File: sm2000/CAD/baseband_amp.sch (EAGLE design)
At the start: 20 parts, among them Q1 BC548, Q4 BC549

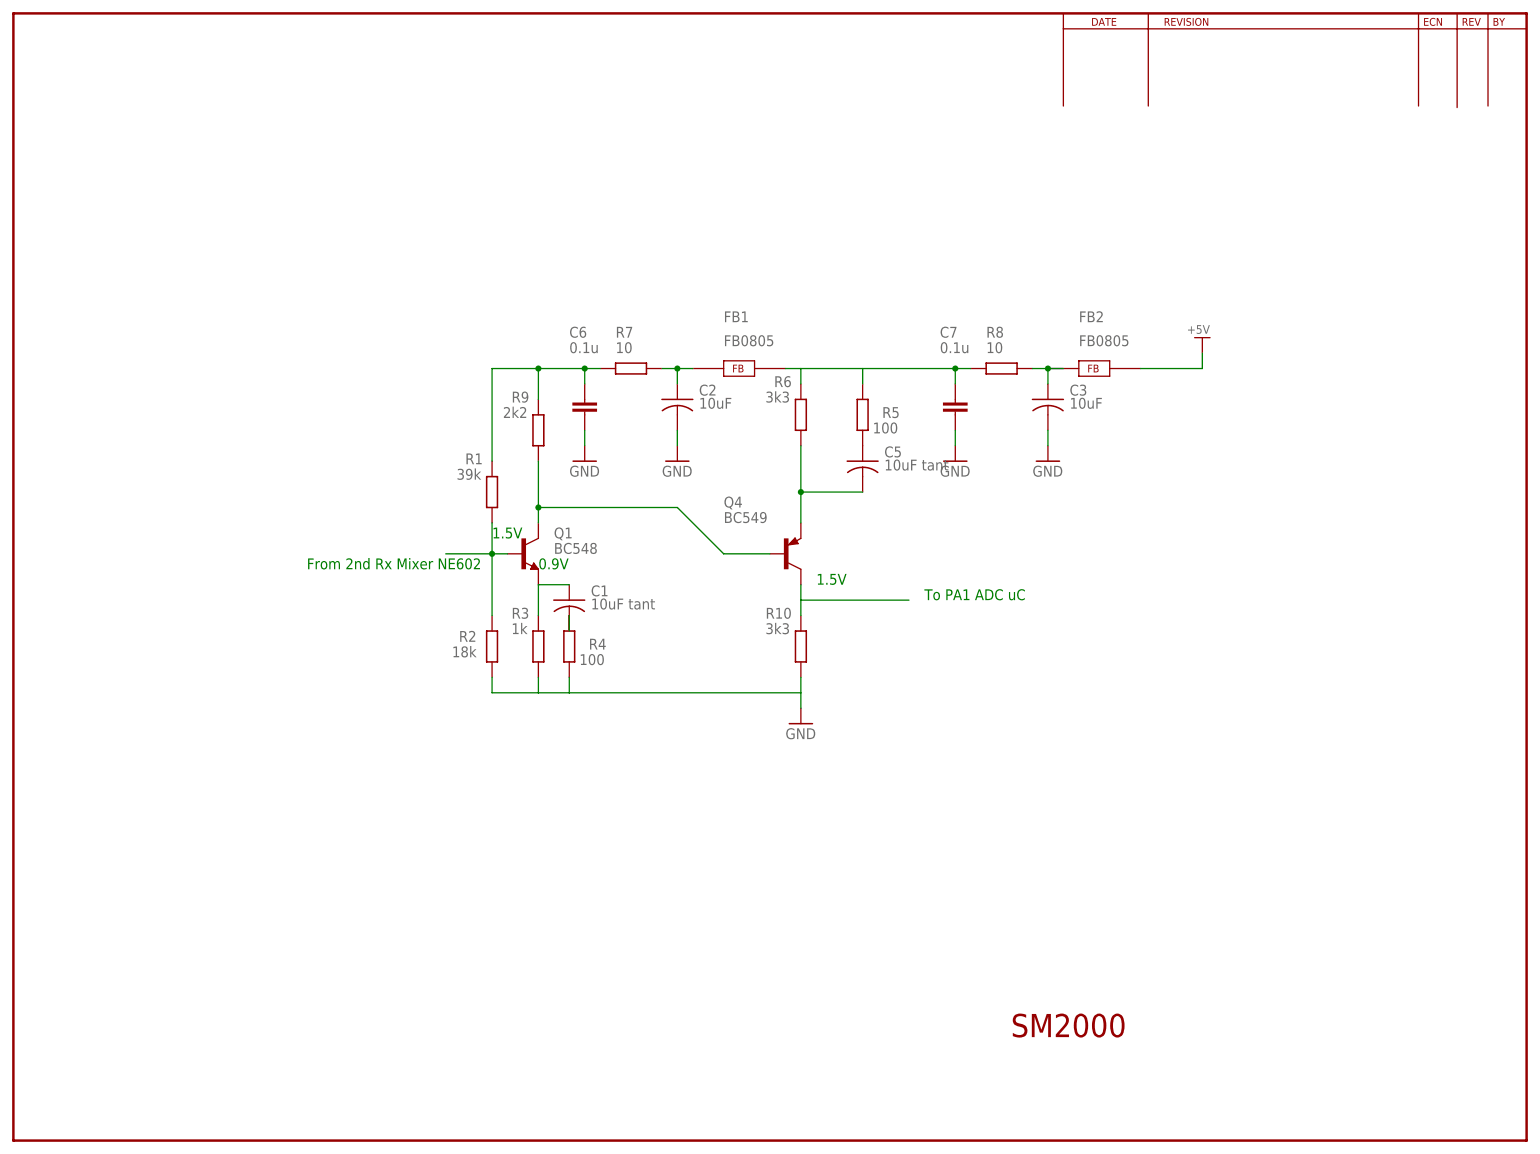
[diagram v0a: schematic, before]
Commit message: COMMIT SM2000 SCHEMATIC, PCB AND ADDED PART DOCS.  RGB
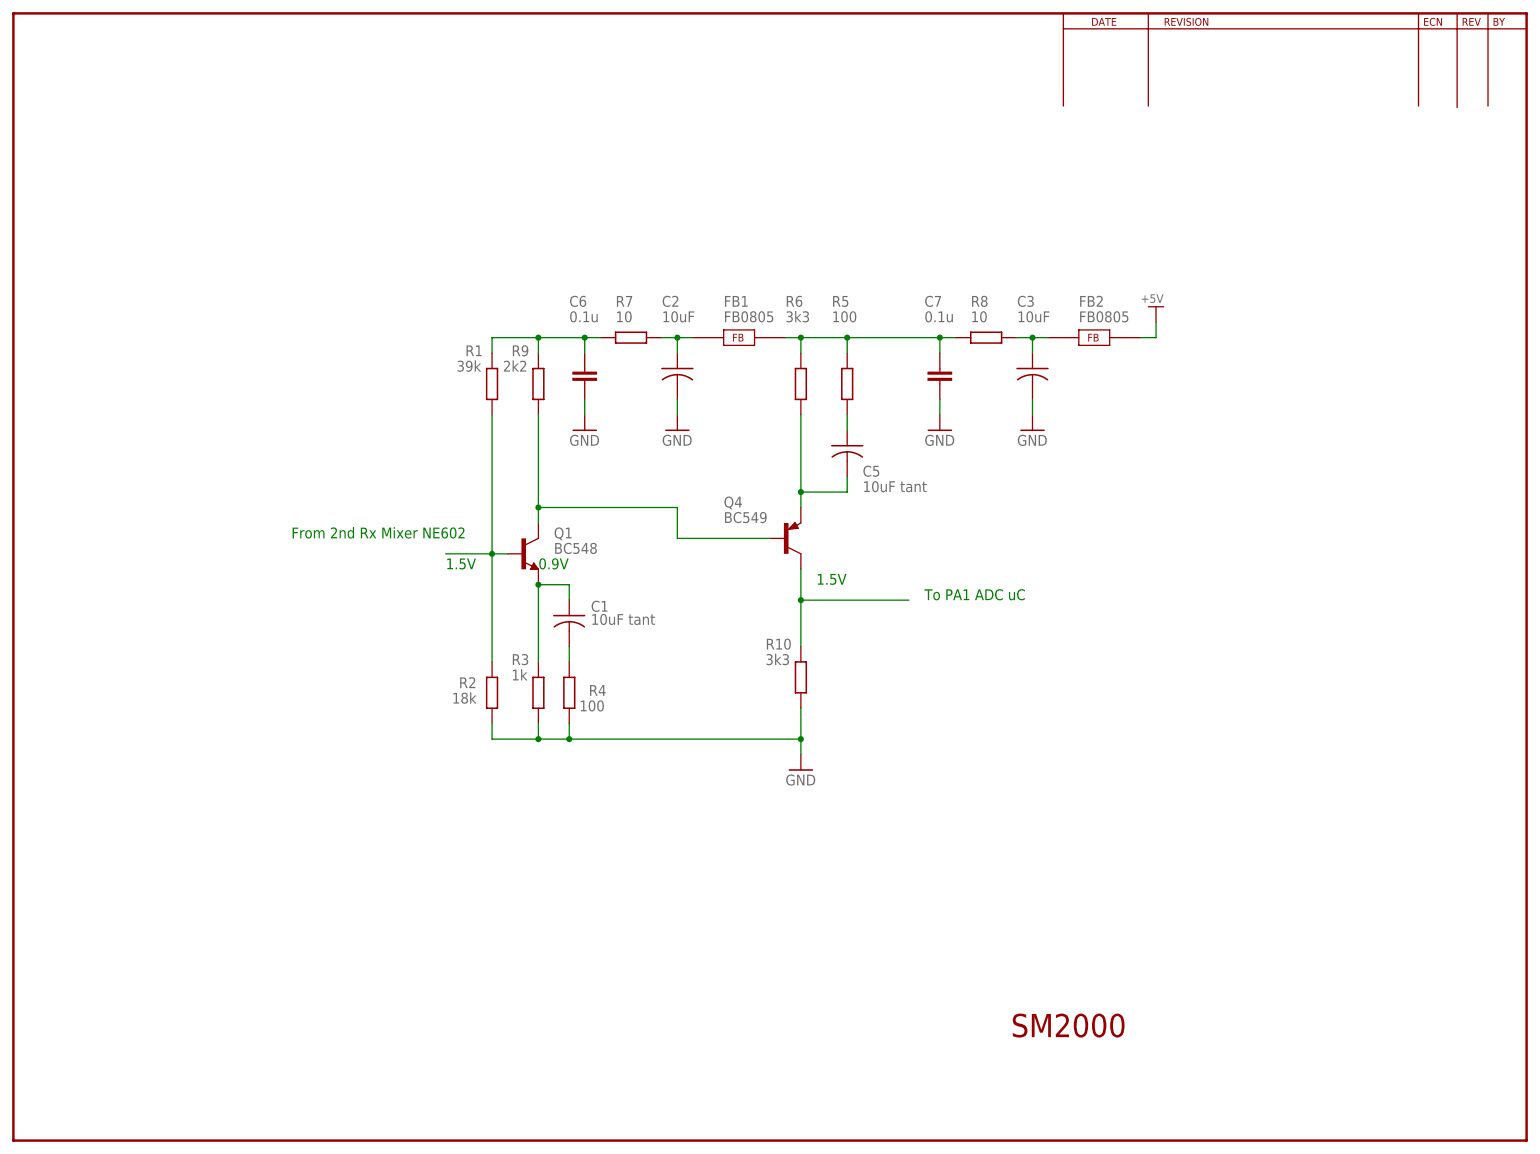
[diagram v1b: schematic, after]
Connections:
- removed net N$11: R2.1, R3.1, R4.1
- net GND: now also R2.1, R3.1, R4.1
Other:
- moved on the sheet: C1, C2, C3, C5, C6, C7, FB1, FB2, Q4, R1, R10, R2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
